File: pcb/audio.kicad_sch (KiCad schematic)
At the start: 0 parts

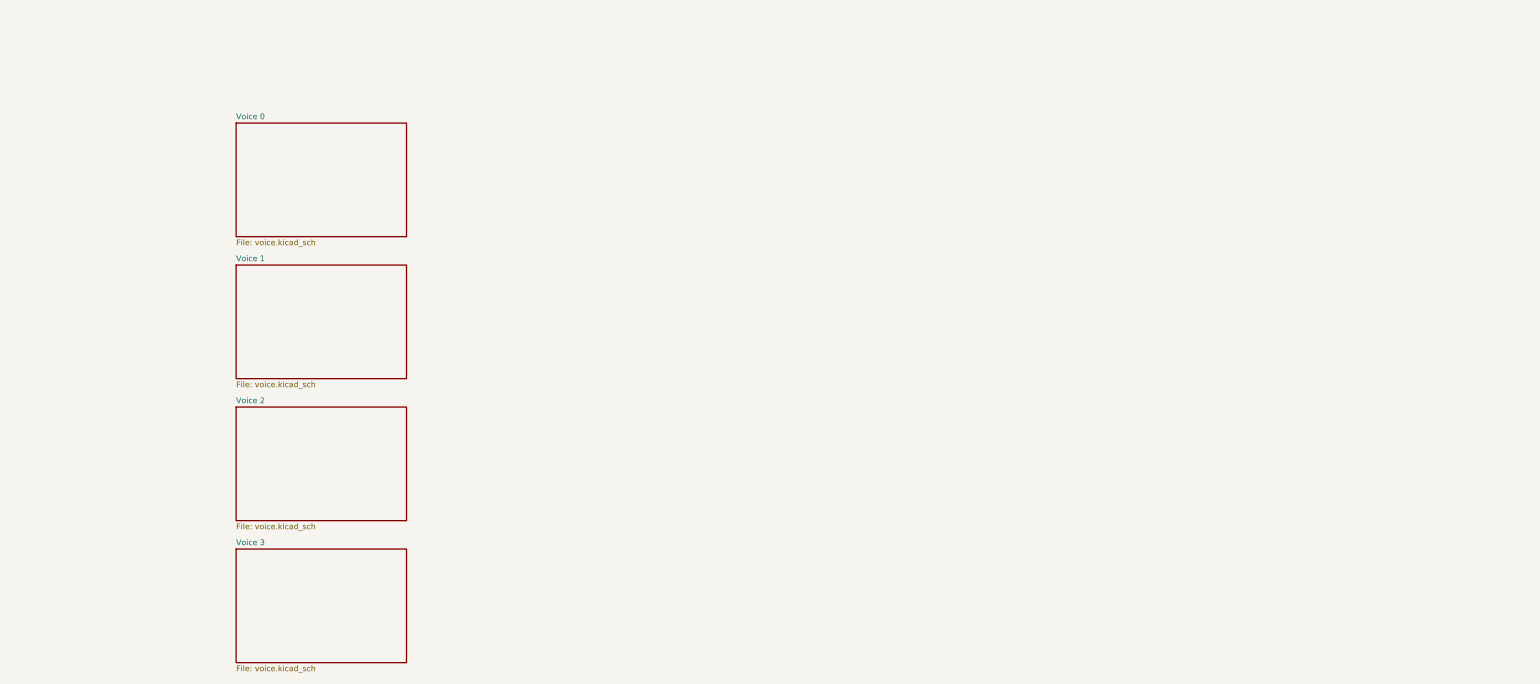
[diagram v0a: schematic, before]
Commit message: WIP schematic
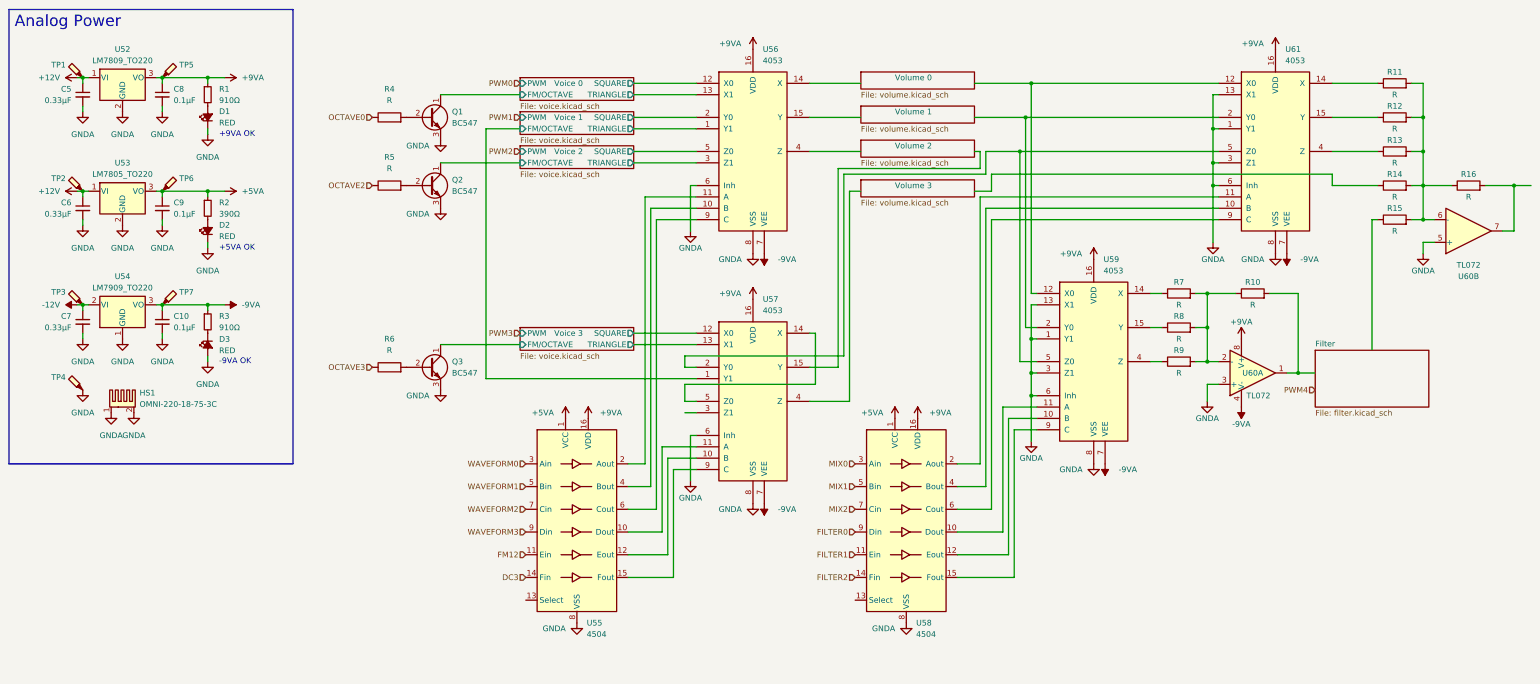
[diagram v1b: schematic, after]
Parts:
- added C10, C8, C9: 0.1µF, symbol Device:C_Small
- added C5, C6, C7: 0.33µF, symbol Device:C_Small
- added D1, D2, D3: RED, symbol Device:LED_Small_Filled
- added HS1: OMNI-220-18-75-3C, symbol Mechanical:Heatsink_Pad_2Pin
- added Q1, Q2, Q3: BC547, Package_TO_SOT_THT:TO-92_Inline, symbol Transistor_BJT:BC547
- added R1, R3: 910Ω, symbol Device:R_Small
- added R10, R11, R12, R13, R14, R15, R16, R4, R5, R6, R7, R8, R9: R, symbol Device:R
- added R2: 390Ω, symbol Device:R_Small
- added TP1, TP2, TP3, TP4, TP5, TP6, TP7: TestPoint_Probe, symbol Connector:TestPoint_Probe
- added U52: LM7809_TO220, Package_TO_SOT_THT:TO-220-3_Vertical, symbol Regulator_Linear:LM7809_TO220
- added U53: LM7805_TO220, Package_TO_SOT_THT:TO-220-3_Vertical, symbol Regulator_Linear:LM7805_TO220
- added U54: LM7909_TO220, Package_TO_SOT_THT:TO-220-3_Vertical, symbol Regulator_Linear:LM7909_TO220
- added U55, U58: 4504, symbol 4xxx:4504
- added U56, U57, U59, U61: 4053, symbol 4xxx:4053
- added U60: TL072, symbol Amplifier_Operational:TL072
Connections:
- new net: R11.1, U61.14 (X)
- new net: R11.2, R12.2, R13.2, R14.2, R15.2, R16.1, U60.6 (-)
- new net: Q3.2 (B), R6.2
- new net: D2.2 (A), R2.2
- new net: Q2.2 (B), R5.2
- new net: Q1.2 (B), R4.2
- new net: D1.2 (A), R1.2
- new net: U58.12 (Eout), U59.10 (B)
- new net: U58.10 (Dout), U59.11 (A)
- new net: U59.12 (X0), U61.12 (X0)
- new net: R7.1, U59.14 (X)
- new net: R8.1, U59.15 (Y)
- new net: U59.2 (Y0), U61.2 (Y0)
- new net: R9.1, U59.4 (Z)
- new net: U57.2 (Y0), U59.5 (Z0), U61.5 (Z0)
- new net: U58.15 (Fout), U59.9 (C)
- new net: R10.1, R7.2, R8.2, R9.2, U60.2 (-)
- new net: U55.10 (Dout), U57.11 (A)
- new net: U55.12 (Eout), U57.10 (B)
- new net: U55.15 (Fout), U57.9 (C)
- new net: U55.2 (Aout), U56.11 (A)
- new net: U55.4 (Bout), U56.10 (B)
- new net: U55.6 (Cout), U56.9 (C)
- new net: U58.4 (Bout), U61.10 (B)
- new net: U58.2 (Aout), U61.11 (A)
- new net: R12.1, U61.15 (Y)
- new net: R13.1, U61.4 (Z)
- new net: U58.6 (Cout), U61.9 (C)
- new net: D3.1 (K), R3.2
- new net: R10.2, U60.1
- new net: R16.2, U60.7
- new net: U57.14 (X), U57.5 (Z0)
- new net +12V: C5.1, C6.1, TP1.1, TP2.1, U52.1 (VI), U53.1 (VI)
- new net +5VA: C9.1, R2.1, TP6.1, U53.3 (VO), U55.1 (VCC), U58.1 (VCC)
- new net +9VA: C8.1, R1.1, TP5.1, U52.3 (VO), U55.16 (VDD), U56.16 (VDD), U57.16 (VDD), U58.16 (VDD), U59.16 (VDD), U60.8 (V+), U61.16 (VDD)
- new net -12V: C7.1, TP3.1, U54.2 (VI)
- new net -9VA: C10.1, R3.1, TP7.1, U54.3 (VO), U56.7 (VEE), U57.7 (VEE), U59.7 (VEE), U60.4 (V-), U61.7 (VEE)
- new net DC3: U55.14 (Fin)
- new net FILTER0: U58.9 (Din)
- new net FILTER1: U58.11 (Ein)
- new net FILTER2: U58.14 (Fin)
- new net FM12: U55.11 (Ein)
- new net GNDA: C10.2, C5.2, C6.2, C7.2, C8.2, C9.2, D1.1 (K), D2.1 (K), D3.2 (A), HS1.1, HS1.2, Q1.3 (E), Q2.3 (E), Q3.3 (E), TP4.1, U52.2 (GND), U53.2 (GND), U54.1 (GND), U55.8 (VSS), U56.6 (Inh), U56.8 (VSS), U57.6 (Inh), U57.8 (VSS), U58.8 (VSS), U59.1 (Y1), U59.13 (X1), U59.3 (Z1), U59.6 (Inh), U59.8 (VSS), U60.3 (+), U60.5 (+), U61.1 (Y1), U61.13 (X1), U61.3 (Z1), U61.6 (Inh), U61.8 (VSS)
- new net MIX0: U58.3 (Ain)
- new net MIX1: U58.5 (Bin)
- new net MIX2: U58.7 (Cin)
- new net OCTAVE0: R4.1
- new net OCTAVE2: R5.1
- new net OCTAVE3: R6.1
- new net Voice 0/FM/OCTAVE: Q1.1 (C)
- new net Voice 0/SQUARE: U56.12 (X0)
- new net Voice 0/TRIANGLE: U56.13 (X1)
- new net Voice 1/FM/OCTAVE: U57.1 (Y1)
- new net Voice 1/SQUARE: U56.2 (Y0)
- new net Voice 1/TRIANGLE: U56.1 (Y1)
- new net Voice 2/FM/OCTAVE: Q2.1 (C)
- new net Voice 2/SQUARE: U56.5 (Z0)
- new net Voice 2/TRIANGLE: U56.3 (Z1)
- new net Voice 3/FM/OCTAVE: Q3.1 (C)
- new net Voice 3/SQUARE: U57.12 (X0)
- new net Voice 3/TRIANGLE: U57.13 (X1)
- new net WAVEFORM0: U55.3 (Ain)
- new net WAVEFORM1: U55.5 (Bin)
- new net WAVEFORM2: U55.7 (Cin)
- new net WAVEFORM3: U55.9 (Din)
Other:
- added sheet Filter (filter.kicad_sch)
- added sheet Volume 0 (volume.kicad_sch)
- added sheet Volume 1 (volume.kicad_sch)
- added sheet Volume 2 (volume.kicad_sch)
- added sheet Volume 3 (volume.kicad_sch)
- sheet Voice 0 ports: added FM/OCTAVE, PWM, SQUARE, TRIANGLE; removed none
- sheet Voice 1 ports: added FM/OCTAVE, PWM, SQUARE, TRIANGLE; removed none
- sheet Voice 2 ports: added FM/OCTAVE, PWM, SQUARE, TRIANGLE; removed none
- sheet Voice 3 ports: added FM/OCTAVE, PWM, SQUARE, TRIANGLE; removed none
- note added: "+5VA OK"
- note added: "+9VA OK"
- note added: "-9VA OK"
- note added: "Analog Power"
